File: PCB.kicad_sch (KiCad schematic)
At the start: 15 parts, among them J1 Conector alimentacao servo, J11 Servo, J12 IR1, J13 IR2, J14 Conector LORA, J15 Conector motor esquerdo, J16 Conector motor direito, J17 Conector ultrassonico, J18 LEDs, J2 Conector bluetooth, J3 Conector Acelerometro, J4 ENCO_SW_Esq, J5 HC6, J6 ENCO_SW_Dir

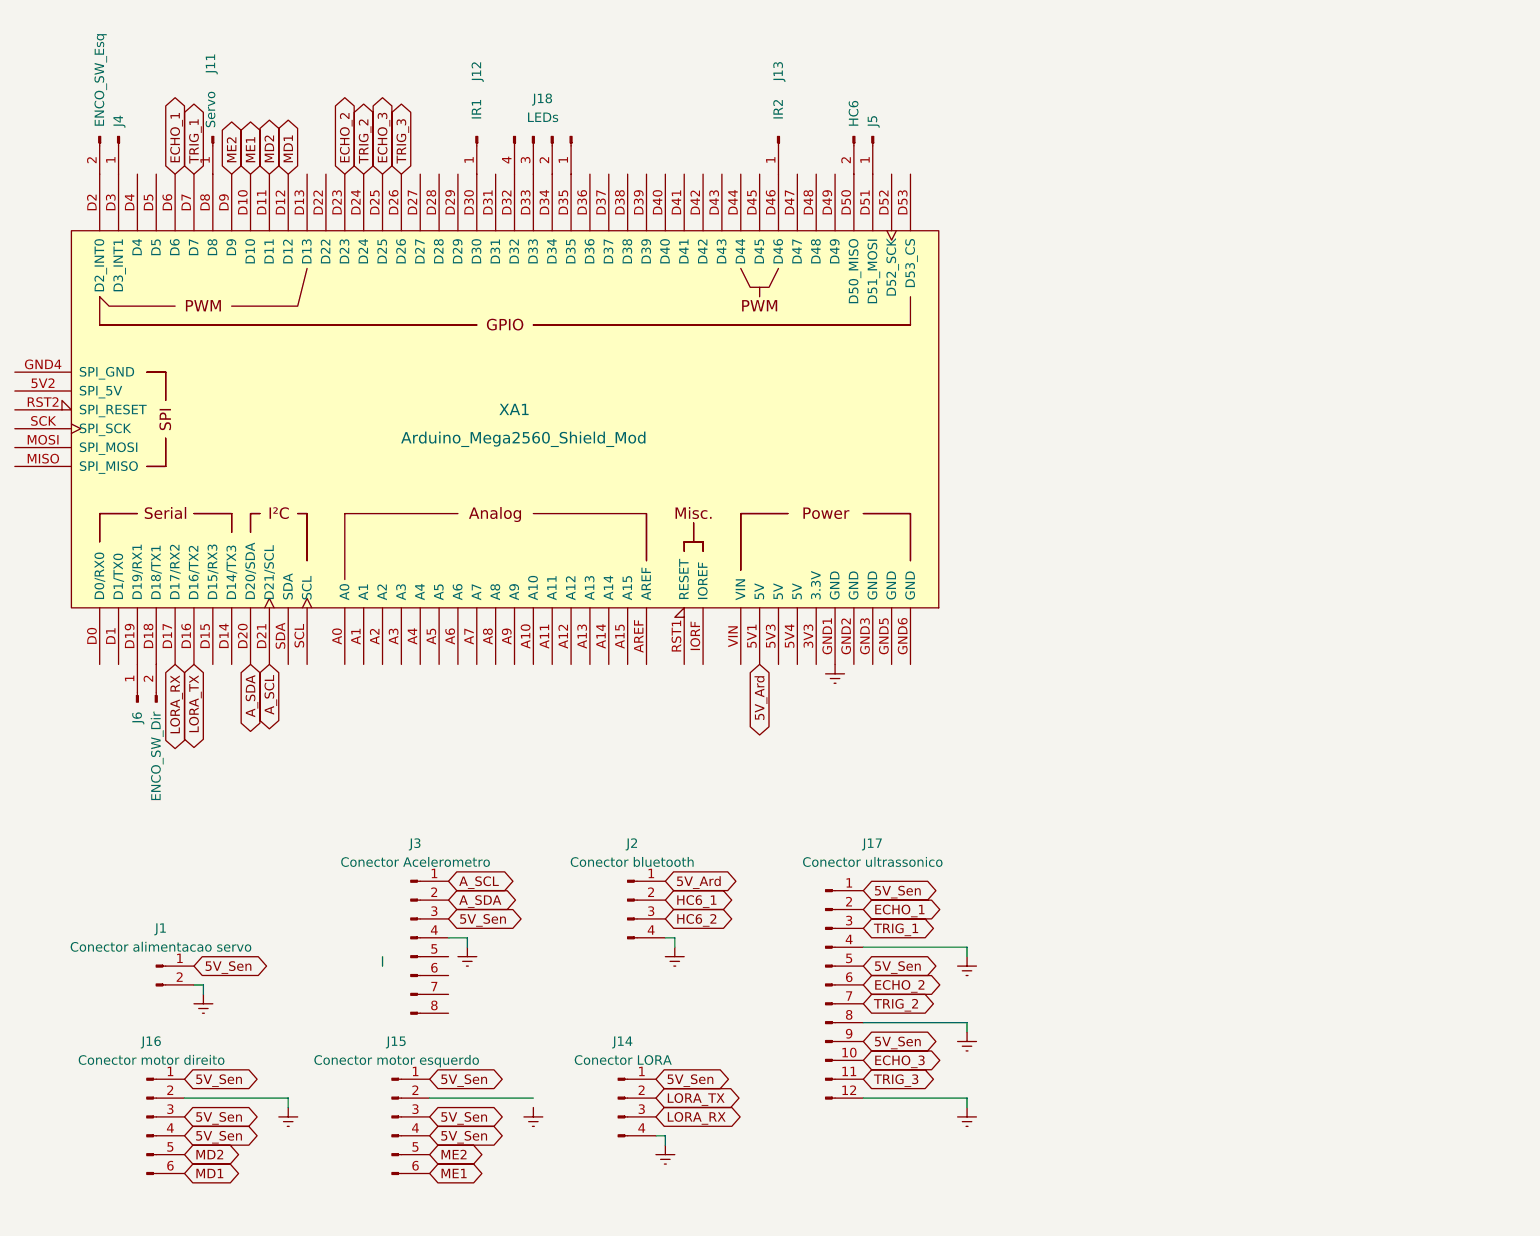
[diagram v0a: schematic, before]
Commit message: feat: criacao do pcb
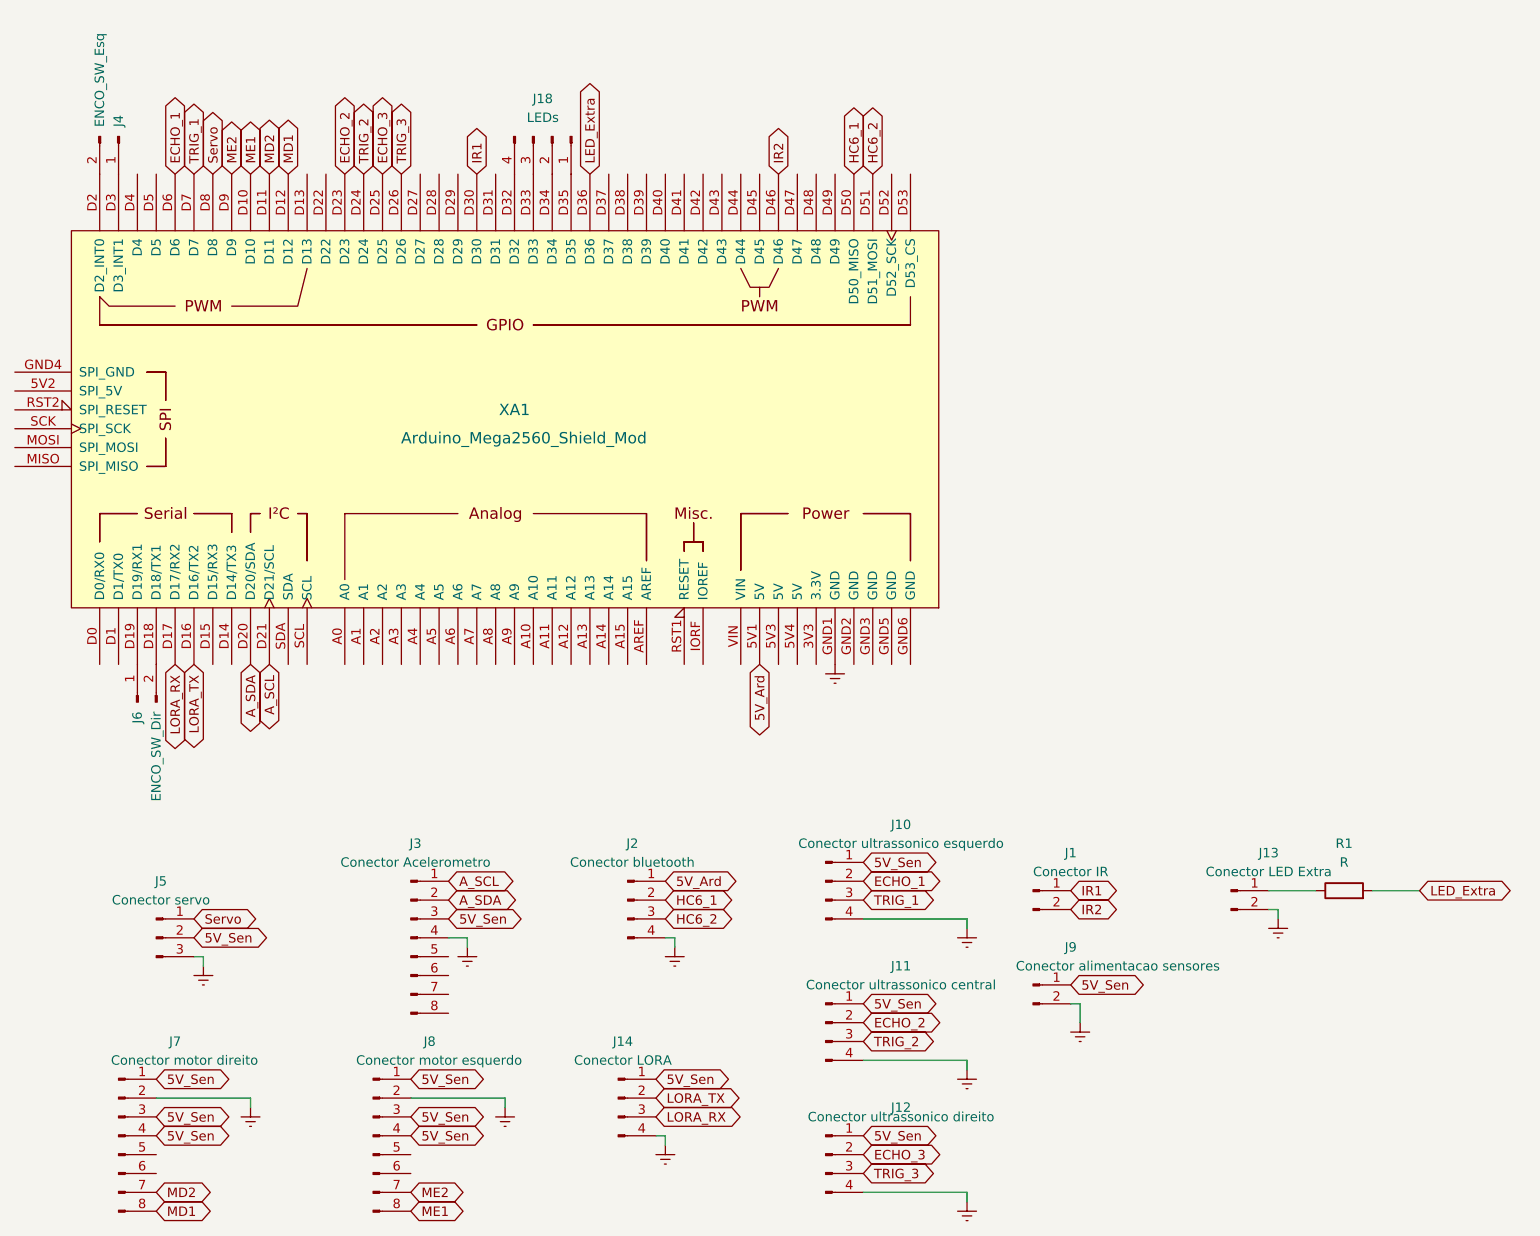
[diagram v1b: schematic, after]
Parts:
- removed J11: Servo, Connector_PinHeader_2.54mm:PinHeader_1x01_P2.54mm_Vertical, symbol Connector:Conn_01x01_Pin
- removed J12: IR1, Connector_PinHeader_2.54mm:PinHeader_1x01_P2.54mm_Vertical, symbol Connector:Conn_01x01_Pin
- removed J13: IR2, Connector_PinHeader_2.54mm:PinHeader_1x01_P2.54mm_Vertical, symbol Connector:Conn_01x01_Pin
- removed J15: Conector motor esquerdo, Connector_PinSocket_2.54mm:PinSocket_2x03_P2.54mm_Vertical, symbol Connector:Conn_01x06_Pin
- removed J16: Conector motor direito, Connector_PinSocket_2.54mm:PinSocket_2x03_P2.54mm_Vertical, symbol Connector:Conn_01x06_Pin
- removed J17: Conector ultrassonico, Connector_PinSocket_2.54mm:PinSocket_2x06_P2.54mm_Vertical, symbol Connector:Conn_01x12_Pin
- removed J5: HC6, Connector_PinSocket_2.54mm:PinSocket_1x02_P2.54mm_Vertical, symbol Connector:Conn_01x02_Pin
- added J10: Conector ultrassonico esquerdo, Connector_JST:JST_XH_B4B-XH-A_1x04_P2.50mm_Vertical, symbol Connector:Conn_01x04_Pin
- added J11: Conector ultrassonico central, Connector_JST:JST_XH_B4B-XH-A_1x04_P2.50mm_Vertical, symbol Connector:Conn_01x04_Pin
- added J12: Conector ultrassonico direito, Connector_JST:JST_XH_B4B-XH-A_1x04_P2.50mm_Vertical, symbol Connector:Conn_01x04_Pin
- added J13: Conector LED Extra, Connector_JST:JST_XH_B2B-XH-A_1x02_P2.50mm_Vertical, symbol Connector:Conn_01x02_Pin
- added J5: Conector servo, TerminalBlock_Phoenix:TerminalBlock_Phoenix_MKDS-1,5-3_1x03_P5.00mm_Horizontal, symbol Connector:Conn_01x03_Pin
- added J7: Conector motor direito, Connector_PinSocket_2.54mm:PinSocket_2x04_P2.54mm_Vertical, symbol Connector:Conn_01x08_Pin
- added J8: Conector motor esquerdo, Connector_PinSocket_2.54mm:PinSocket_2x04_P2.54mm_Vertical, symbol Connector:Conn_01x08_Pin
- added J9: Conector alimentacao sensores, TerminalBlock_Phoenix:TerminalBlock_Phoenix_MKDS-1,5-2_1x02_P5.00mm_Horizontal, symbol Connector:Conn_01x02_Pin
- added R1: R, Resistor_THT:R_Axial_DIN0207_L6.3mm_D2.5mm_P10.16mm_Horizontal, symbol Device:R
- J1: value Conector alimentacao servo -> Conector IR; footprint TerminalBlock_Phoenix:TerminalBlock_Phoenix_MKDS-1,5-2_1x02_P5.00mm_Horizontal -> Connector_JST:JST_XH_B2B-XH-A_1x02_P2.50mm_Vertical
- J14: footprint TerminalBlock_Phoenix:TerminalBlock_Phoenix_MKDS-1,5-4_1x04_P5.00mm_Horizontal -> Connector_JST:JST_XH_B4B-XH-A_1x04_P2.50mm_Vertical
- XA1: footprint PCM_arduino-library:Arduino_Mega2560_R3_Shield -> PCM_arduino-library:Arduino_Mega2560_R3_Shield_Sem_furo
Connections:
- net 5V_Sen: now also J10.1 (Pin_1), J11.1 (Pin_1), J12.1 (Pin_1), J5.2 (Pin_2), J7.1 (Pin_1), J7.3 (Pin_3), J7.4 (Pin_4), J8.1 (Pin_1), J8.3 (Pin_3), J8.4 (Pin_4), J9.1 (Pin_1); no longer J1.1 (Pin_1)
- net ECHO_1: now also J10.2 (Pin_2)
- net ECHO_2: now also J11.2 (Pin_2)
- net ECHO_3: now also J12.2 (Pin_2)
- net Earth: now also J10.4 (Pin_4), J11.4 (Pin_4), J12.4 (Pin_4), J13.2 (Pin_2), J5.3 (Pin_3), J7.2 (Pin_2), J8.2 (Pin_2), J9.2 (Pin_2); no longer J1.2 (Pin_2)
- net HC6_1: now also XA1.D50 (D50_MISO)
- net HC6_2: now also XA1.D51 (D51_MOSI)
- net MD1: now also J7.8 (Pin_8)
- net MD2: now also J7.7 (Pin_7)
- net ME1: now also J8.8 (Pin_8)
- net ME2: now also J8.7 (Pin_7)
- net TRIG_1: now also J10.3 (Pin_3)
- net TRIG_2: now also J11.3 (Pin_3)
- net TRIG_3: now also J12.3 (Pin_3)
- net IR1: now reaches XA1.D30
- net IR1: now also J1.1 (Pin_1)
- net LED_Extra: now reaches XA1.D36
- net LED_Extra: now also R1.2
- net IR2: now reaches XA1.D46
- net IR2: now also J1.2 (Pin_2)
- net Servo: now reaches XA1.D8
- net Servo: now also J5.1 (Pin_1)
- new net: J13.1 (Pin_1), R1.1
